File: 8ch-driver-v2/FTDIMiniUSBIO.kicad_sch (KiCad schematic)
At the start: 5 parts, among them J5 CN2, J6 CN3, U18 BD33FC0FP

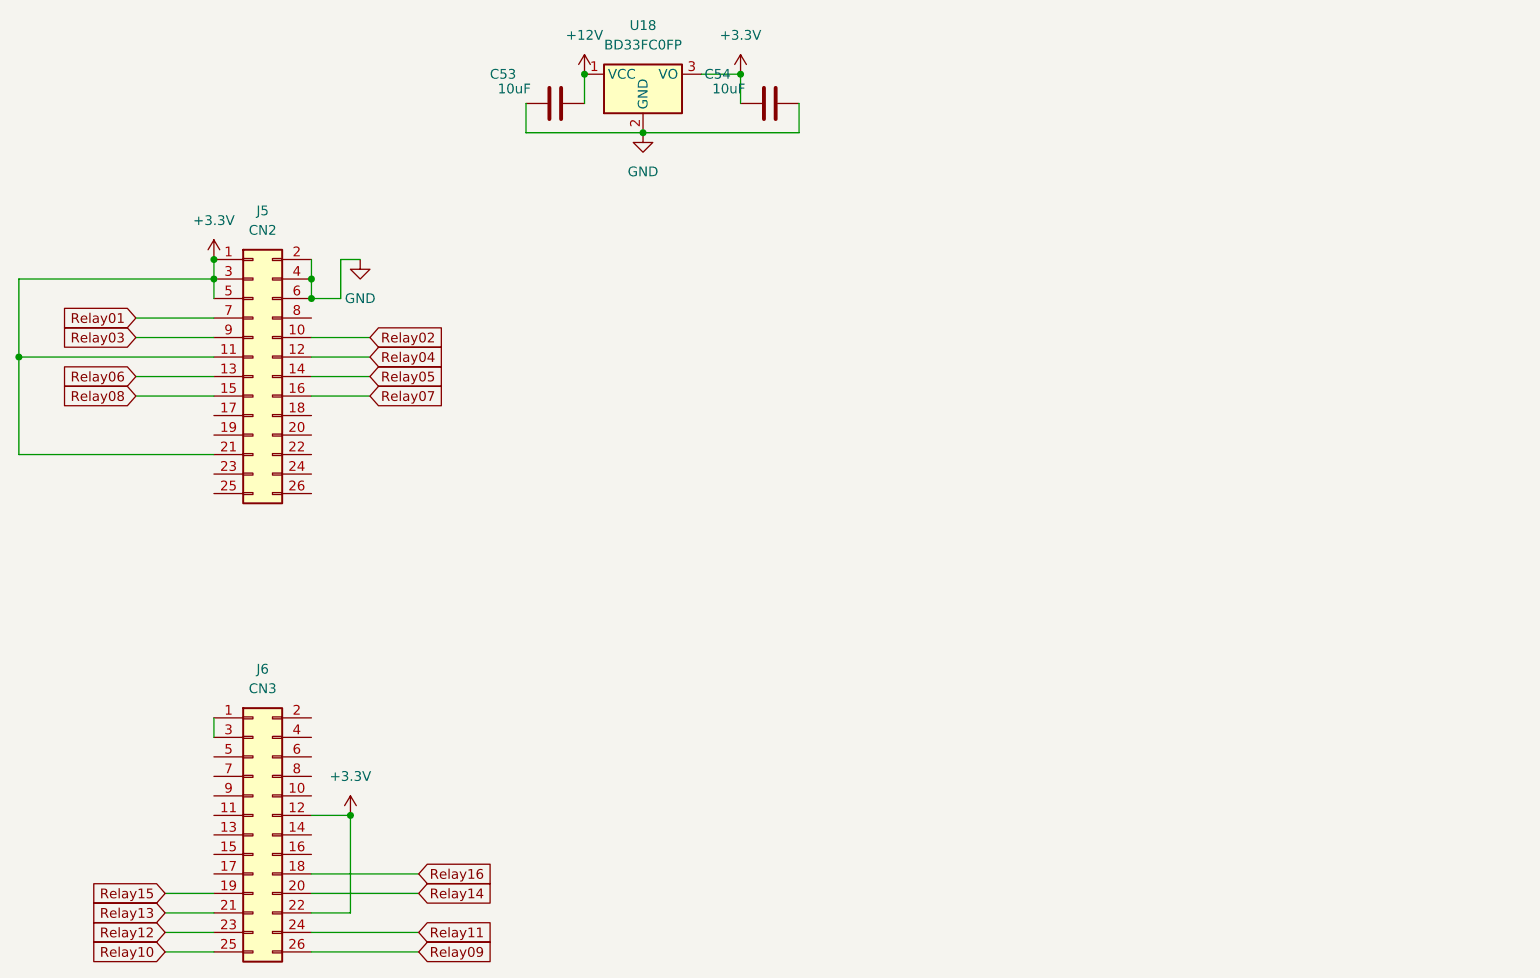
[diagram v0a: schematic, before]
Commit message: progress
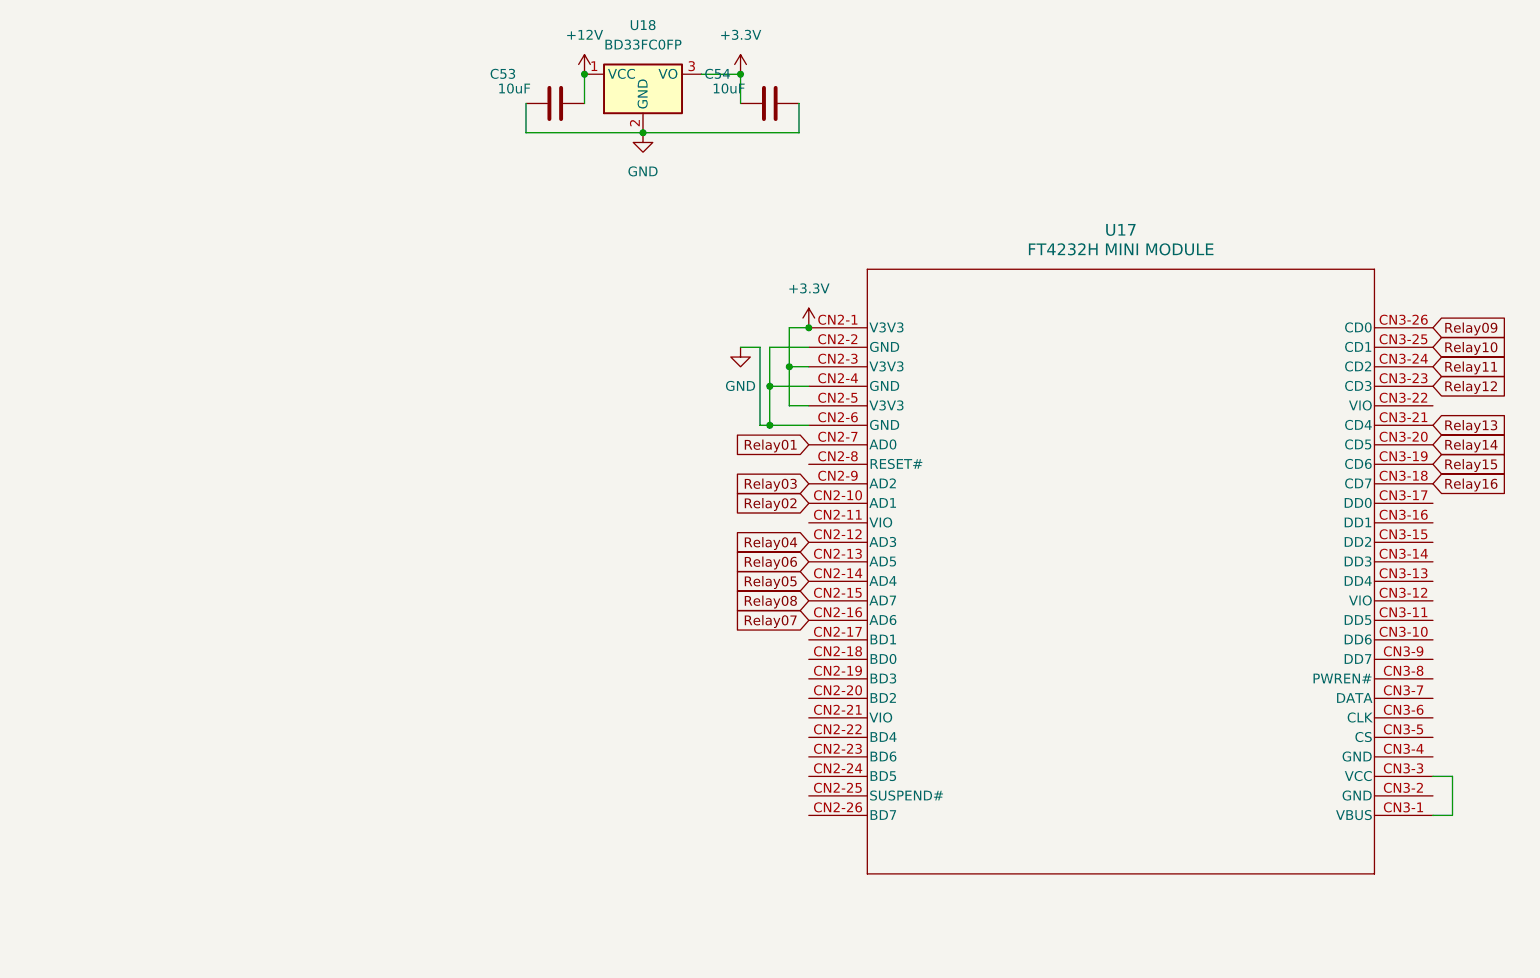
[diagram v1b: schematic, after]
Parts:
- removed J5: CN2, symbol Connector_Generic:Conn_02x13_Odd_Even
- removed J6: CN3, symbol Connector_Generic:Conn_02x13_Odd_Even
- added U17: FT4232H MINI MODULE, FT4232H_FTD, symbol 2024-07-09_22-42-21:FT4232H_MINI_MODULE
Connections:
- net +3.3V: now also U17.CN2-1 (V3V3), U17.CN2-3 (V3V3), U17.CN2-5 (V3V3)
- net GND: now also U17.CN2-2 (GND), U17.CN2-4 (GND), U17.CN2-6 (GND)
- net Relay01: now also U17.CN2-7 (AD0)
- net Relay02: now also U17.CN2-10 (AD1)
- net Relay03: now also U17.CN2-9 (AD2)
- net Relay04: now also U17.CN2-12 (AD3)
- net Relay05: now also U17.CN2-14 (AD4)
- net Relay06: now also U17.CN2-13 (AD5)
- net Relay07: now also U17.CN2-16 (AD6)
- net Relay08: now also U17.CN2-15 (AD7)
- net Relay09: now also U17.CN3-26 (CD0)
- net Relay10: now also U17.CN3-25 (CD1)
- net Relay11: now also U17.CN3-24 (CD2)
- net Relay12: now also U17.CN3-23 (CD3)
- net Relay13: now also U17.CN3-21 (CD4)
- net Relay14: now also U17.CN3-20 (CD5)
- net Relay15: now also U17.CN3-19 (CD6)
- net Relay16: now also U17.CN3-18 (CD7)
- new net: U17.CN3-1 (VBUS), U17.CN3-3 (VCC)
